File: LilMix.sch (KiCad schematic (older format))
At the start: 0 parts

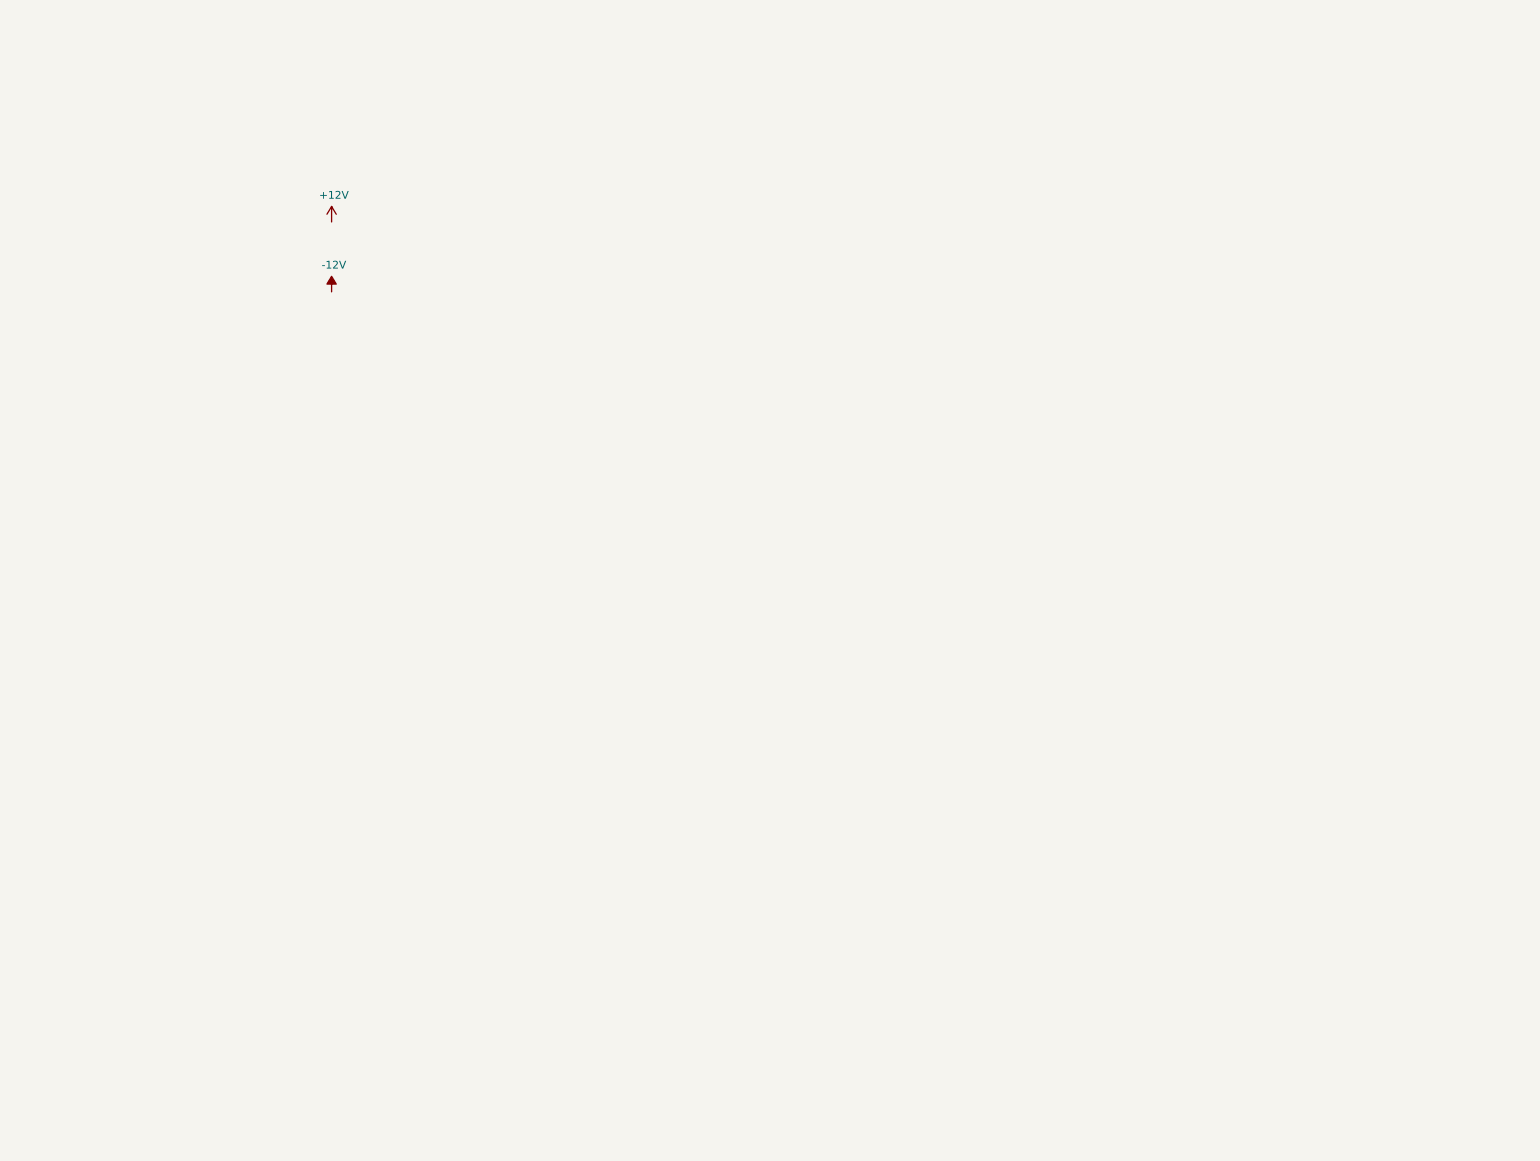
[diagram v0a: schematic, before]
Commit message: Initial version of circuit
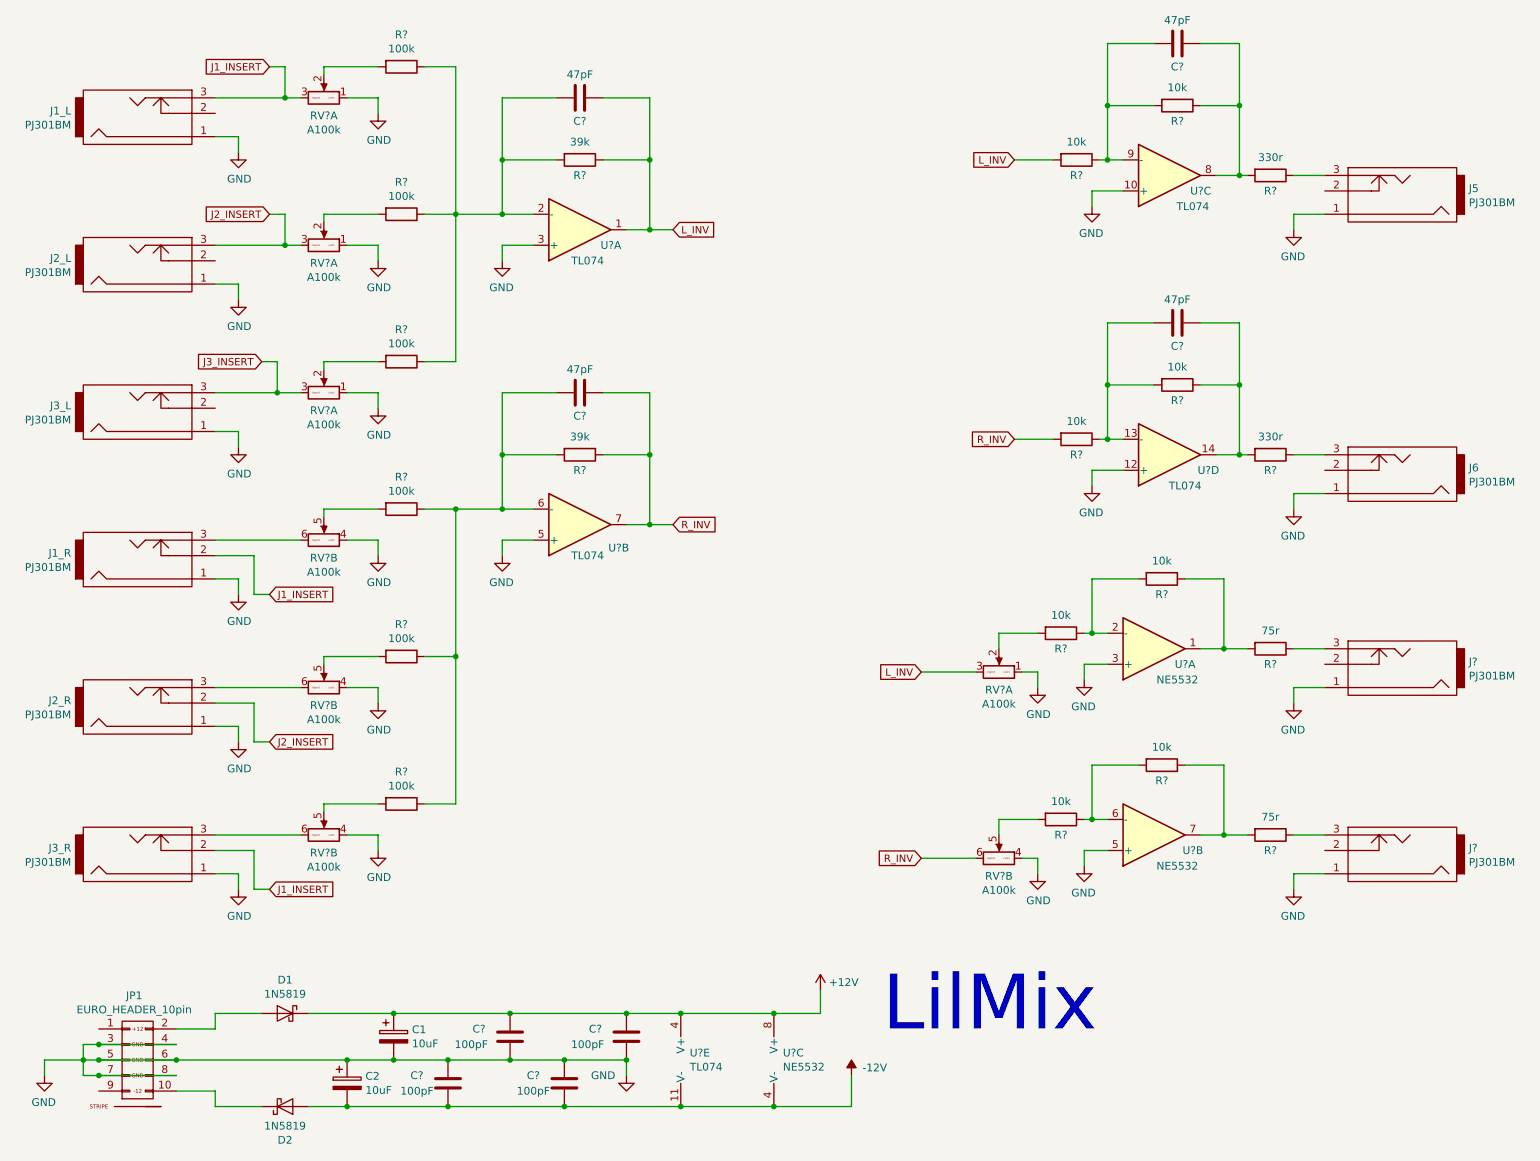
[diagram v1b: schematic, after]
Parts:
- added C1, C2: 10uF, symbol Device:CP
- added C? (x4): 47pF, symbol 4ms-passives:C
- added C? (x4): 100pF, symbol 4ms-passives:C
- added D1, D2: 1N5819, symbol 4ms-passives:D_Schottky
- added J1_L, J1_R, J2_L, J2_R, J3_L, J3_R, J5, J6, J? (x2): PJ301BM, Eurocad:EighthInch_PJ301BM_CC_FIXED, symbol eurocad:PJ301M-12
- added JP1: EURO_HEADER_10pin, 4ms-footprints:Header_2x05_Pitch2.54mm_TH_-12v_Label, symbol 4ms-headers:EURO_HEADER_10pin
- added R? (x8): 10k, symbol 4ms-passives:R
- added R? (x6): 100k, symbol 4ms-passives:R
- added R? (x2): 330r, symbol 4ms-passives:R
- added R? (x2): 39k, symbol 4ms-passives:R
- added R? (x2): 75r, symbol 4ms-passives:R
- added RV? (x8): A100k, symbol 4ms-mech:POT_DUAL
- added U? (x5): TL074, symbol Amplifier_Operational:TL074
- added U? (x3): NE5532, symbol Amplifier_Operational:NE5532
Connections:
- net +12V: now also C1.1, C?.1, C?.1, D1.1 (K), U?.4 (V+), U?.8 (V+)
- net -12V: now also C2.2, C?.2, C?.2, D2.2 (A), U?.11 (V-), U?.4 (V-)
- new net: D2.1 (K), JP1.10 (-12V)
- new net: D1.2 (A), JP1.2 (+12V)
- new net: C?.2, R?.1, R?.2, U?.13 (-)
- new net: C?.2, R?.1, R?.1, R?.1, R?.2, U?.2 (-)
- new net: R?.2, RV?.2 (Center) (x4)
- new net: J1_R.3, RV?.6 (Right)
- new net: J2_R.3, RV?.6 (Right)
- new net: J3_R.3, RV?.6 (Right)
- new net: C?.2, R?.1, R?.1, R?.1, R?.2, U?.6 (-)
- new net: R?.2, RV?.5 (Center) (x4)
- new net: J5.3, R?.1
- new net: J6.3, R?.1
- new net: C?.1, R?.1, R?.2, U?.8
- new net: C?.1, R?.1, R?.2, U?.14
- new net: C?.2, R?.1, R?.2, U?.9 (-)
- new net: R?.1, R?.2, U?.1
- new net: R?.1, R?.2, U?.2 (-)
- new net: R?.1, R?.2, U?.6 (-)
- new net: R?.1, R?.2, U?.7
- new net: J?.3, R?.1 (x2)
- new net GND: C1.2, C2.1, C?.1, C?.1, C?.2, C?.2, J1_L.1, J1_R.1, J2_L.1, J2_R.1, J3_L.1, J3_R.1, J5.1, J6.1, J?.1, J?.1, JP1.3 (GND), JP1.4 (GND), JP1.5 (GND), JP1.6 (GND), JP1.7 (GND), JP1.8 (GND), RV?.1 (Left), RV?.1 (Left), RV?.1 (Left), RV?.1 (Left), RV?.4 (Left), RV?.4 (Left), RV?.4 (Left), RV?.4 (Left), U?.10 (+), U?.12 (+), U?.3 (+), U?.3 (+), U?.5 (+), U?.5 (+)
- new net J1_INSERT: J1_L.3, J1_R.2, J3_R.2, RV?.3 (Right)
- new net J2_INSERT: J2_L.3, J2_R.2, RV?.3 (Right)
- new net J3_INSERT: J3_L.3, RV?.3 (Right)
- new net L_INV: C?.1, R?.1, R?.2, RV?.3 (Right), U?.1
- new net R_INV: C?.1, R?.1, R?.2, RV?.6 (Right), U?.7
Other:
- note added: "LilMix"
